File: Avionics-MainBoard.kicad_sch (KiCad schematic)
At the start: 0 parts

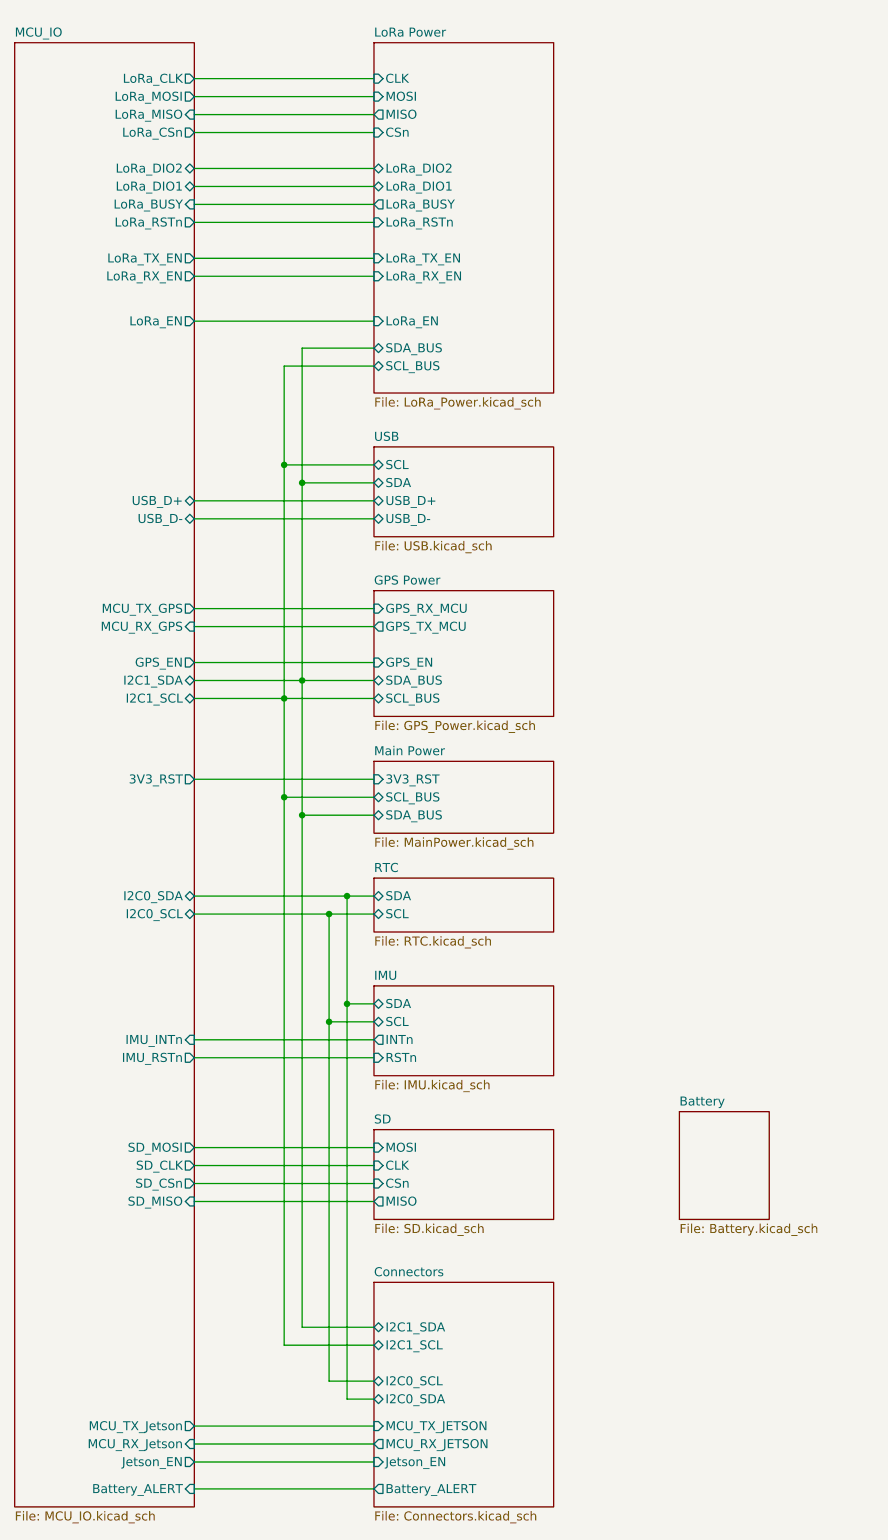
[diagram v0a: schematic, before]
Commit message: temp
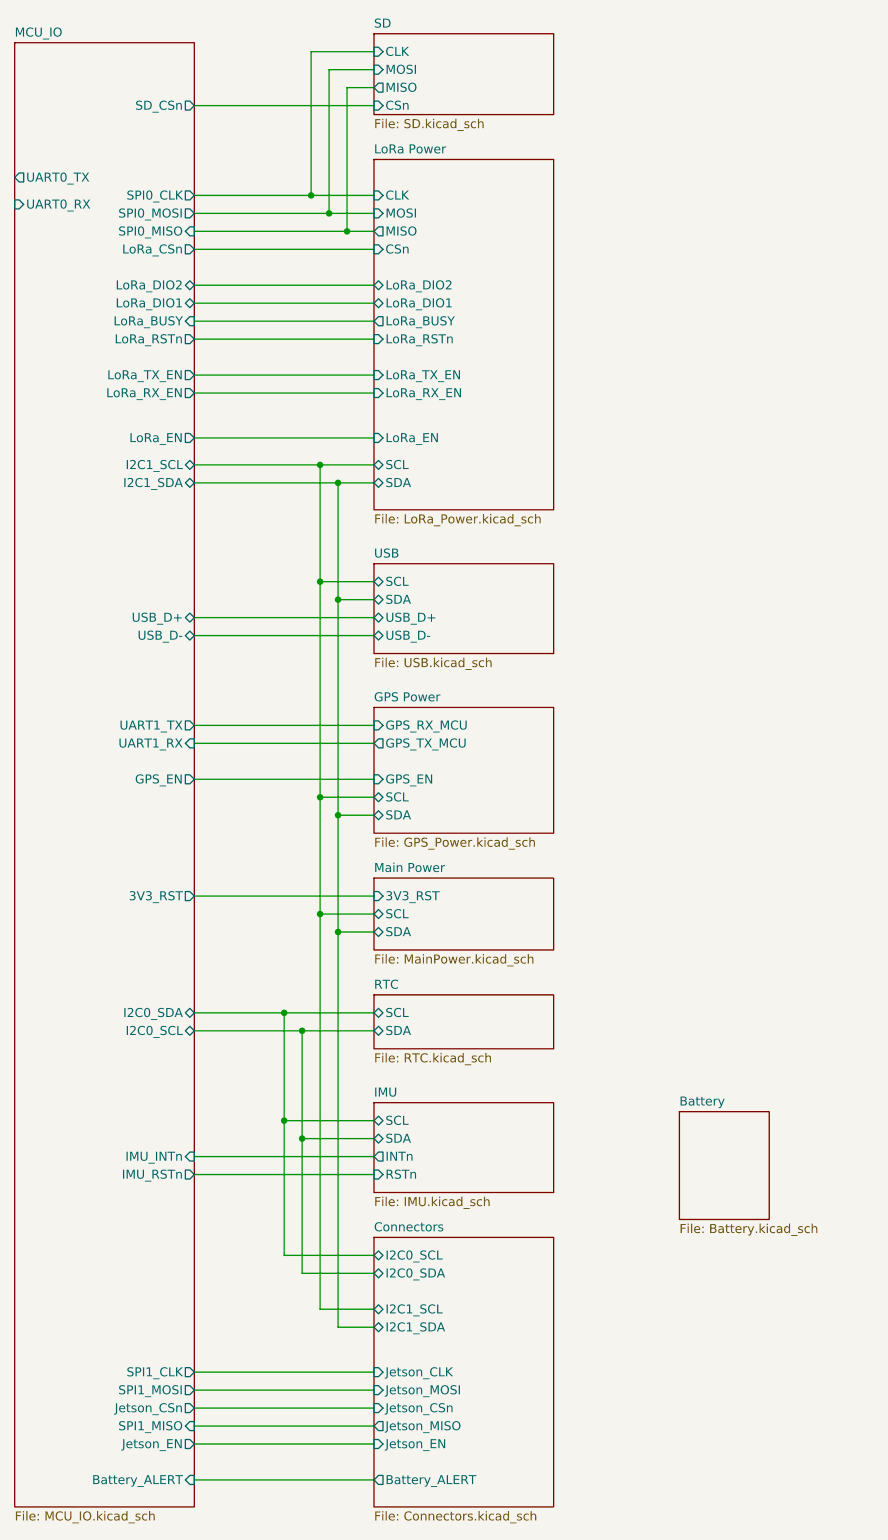
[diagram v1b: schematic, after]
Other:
- sheet Connectors ports: added Jetson_CLK, Jetson_CSn, Jetson_MISO, Jetson_MOSI; removed MCU_RX_JETSON, MCU_TX_JETSON
- sheet GPS Power ports: added SCL, SDA; removed SCL_BUS, SDA_BUS
- sheet LoRa Power ports: added SCL, SDA; removed SCL_BUS, SDA_BUS
- sheet MCU_IO ports: added Jetson_CSn, SPI0_CLK, SPI0_MISO, SPI0_MOSI, SPI1_CLK, SPI1_MISO, SPI1_MOSI, UART0_RX, UART0_TX, UART1_RX, UART1_TX; removed LoRa_CLK, LoRa_MISO, LoRa_MOSI, MCU_RX_GPS, MCU_RX_Jetson, MCU_TX_GPS, MCU_TX_Jetson, SD_CLK, SD_MISO, SD_MOSI
- sheet Main Power ports: added SCL, SDA; removed SCL_BUS, SDA_BUS
